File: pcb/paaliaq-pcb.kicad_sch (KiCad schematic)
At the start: 9 parts, among them J1 SODIMM-200, J2 HDMI_A, U1 W65C816SxP, U3 MCP1727-3302xSN

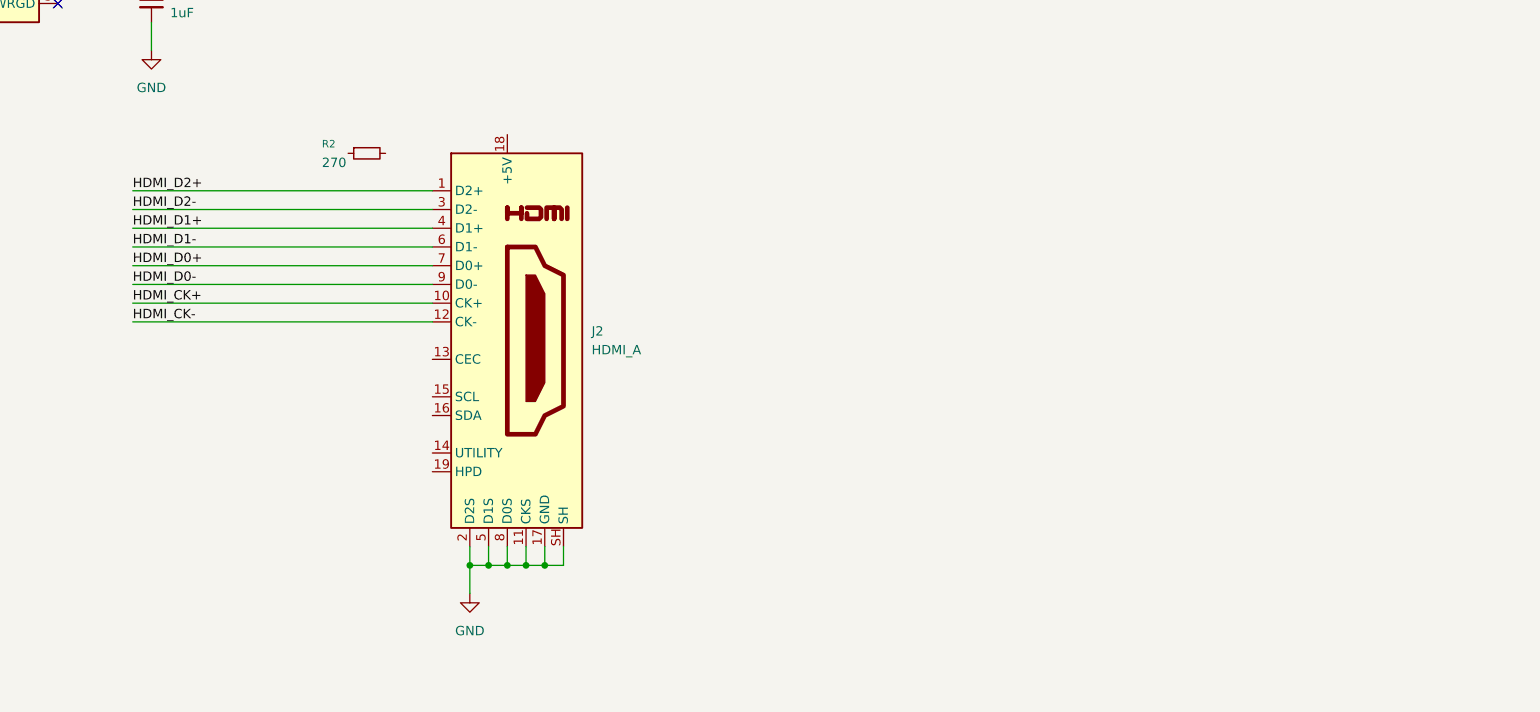
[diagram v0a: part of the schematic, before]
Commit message: wip dvi phy
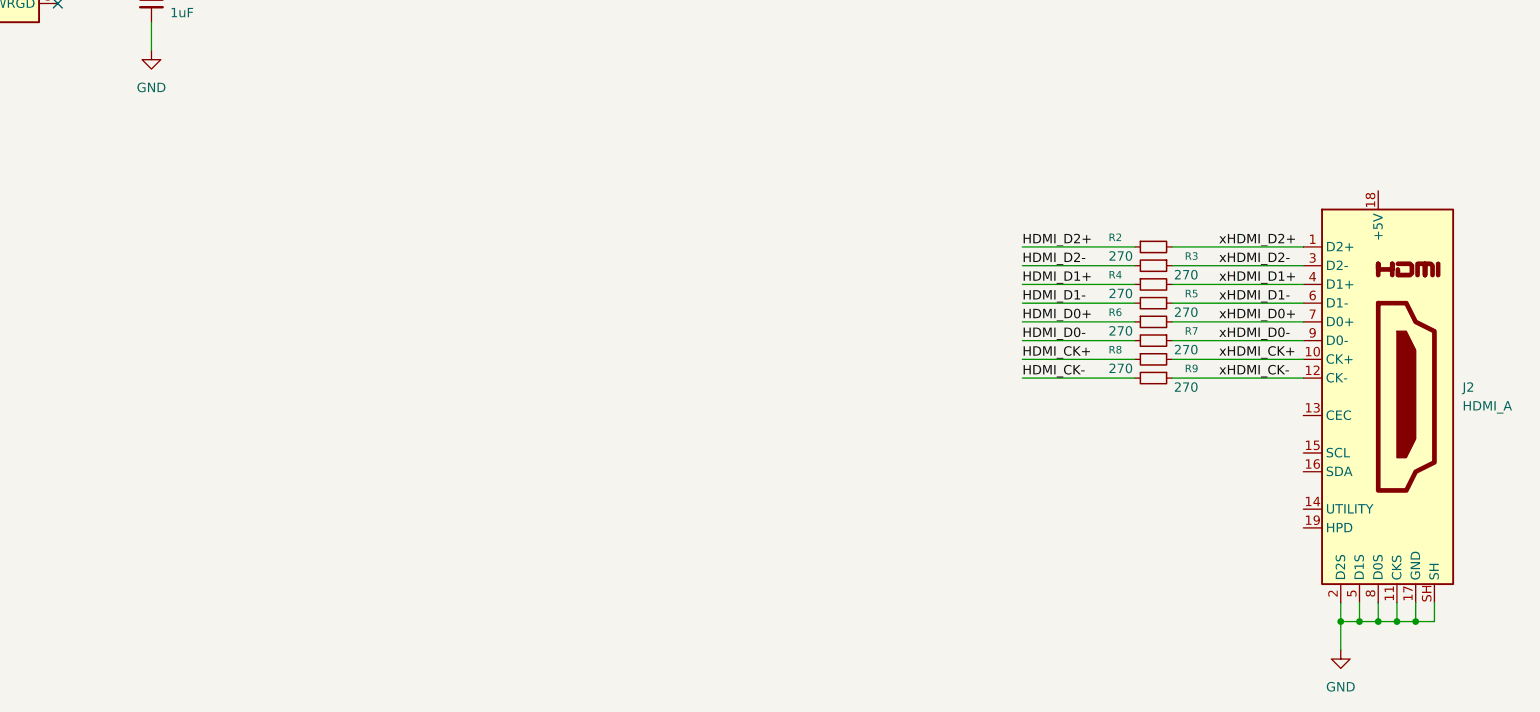
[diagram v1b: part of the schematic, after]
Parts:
- added R3, R4, R5, R6, R7, R8, R9: 270, Resistor_SMD:R_0603_1608Metric_Pad0.98x0.95mm_HandSolder, symbol Device:R_Small
- R2: footprint Resistor_SMD:R_0805_2012Metric_Pad1.20x1.40mm_HandSolder -> Resistor_SMD:R_0603_1608Metric_Pad0.98x0.95mm_HandSolder
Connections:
- net HDMI_CK+: now also R8.1; no longer J2.10 (CK+)
- net HDMI_CK-: now also R9.2; no longer J2.12 (CK-)
- net HDMI_D0+: now also R6.1; no longer J2.7 (D0+)
- net HDMI_D0-: now also R7.2; no longer J2.9 (D0-)
- net HDMI_D1+: now also R4.1; no longer J2.4 (D1+)
- net HDMI_D1-: now also R5.2; no longer J2.6 (D1-)
- net HDMI_D2+: now also R2.1; no longer J2.1 (D2+)
- net HDMI_D2-: now also R3.2; no longer J2.3 (D2-)
- net xHDMI_D2+: now reaches R2.2
- net xHDMI_D2+: now also J2.1 (D2+)
- new net xHDMI_CK+: J2.10 (CK+), R8.2
- new net xHDMI_CK-: J2.12 (CK-), R9.1
- new net xHDMI_D0+: J2.7 (D0+), R6.2
- new net xHDMI_D0-: J2.9 (D0-), R7.1
- new net xHDMI_D1+: J2.4 (D1+), R4.2
- new net xHDMI_D1-: J2.6 (D1-), R5.1
- new net xHDMI_D2-: J2.3 (D2-), R3.1
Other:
- moved on the sheet: J2, R2

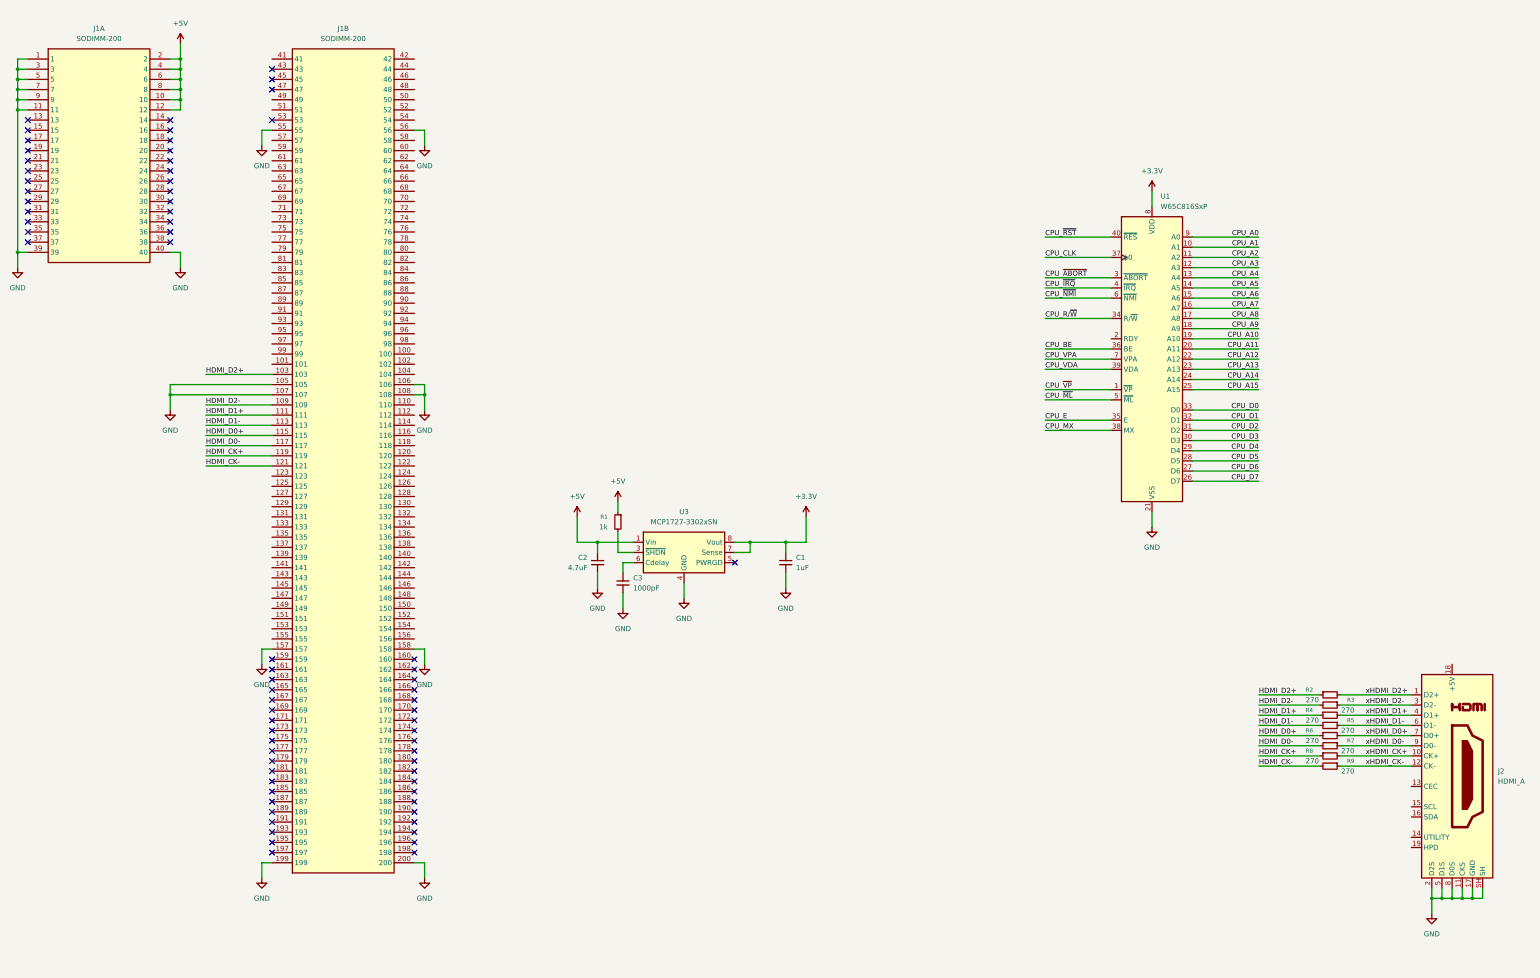
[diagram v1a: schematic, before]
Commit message: wip use resistor arrays and swap pairs and +/-
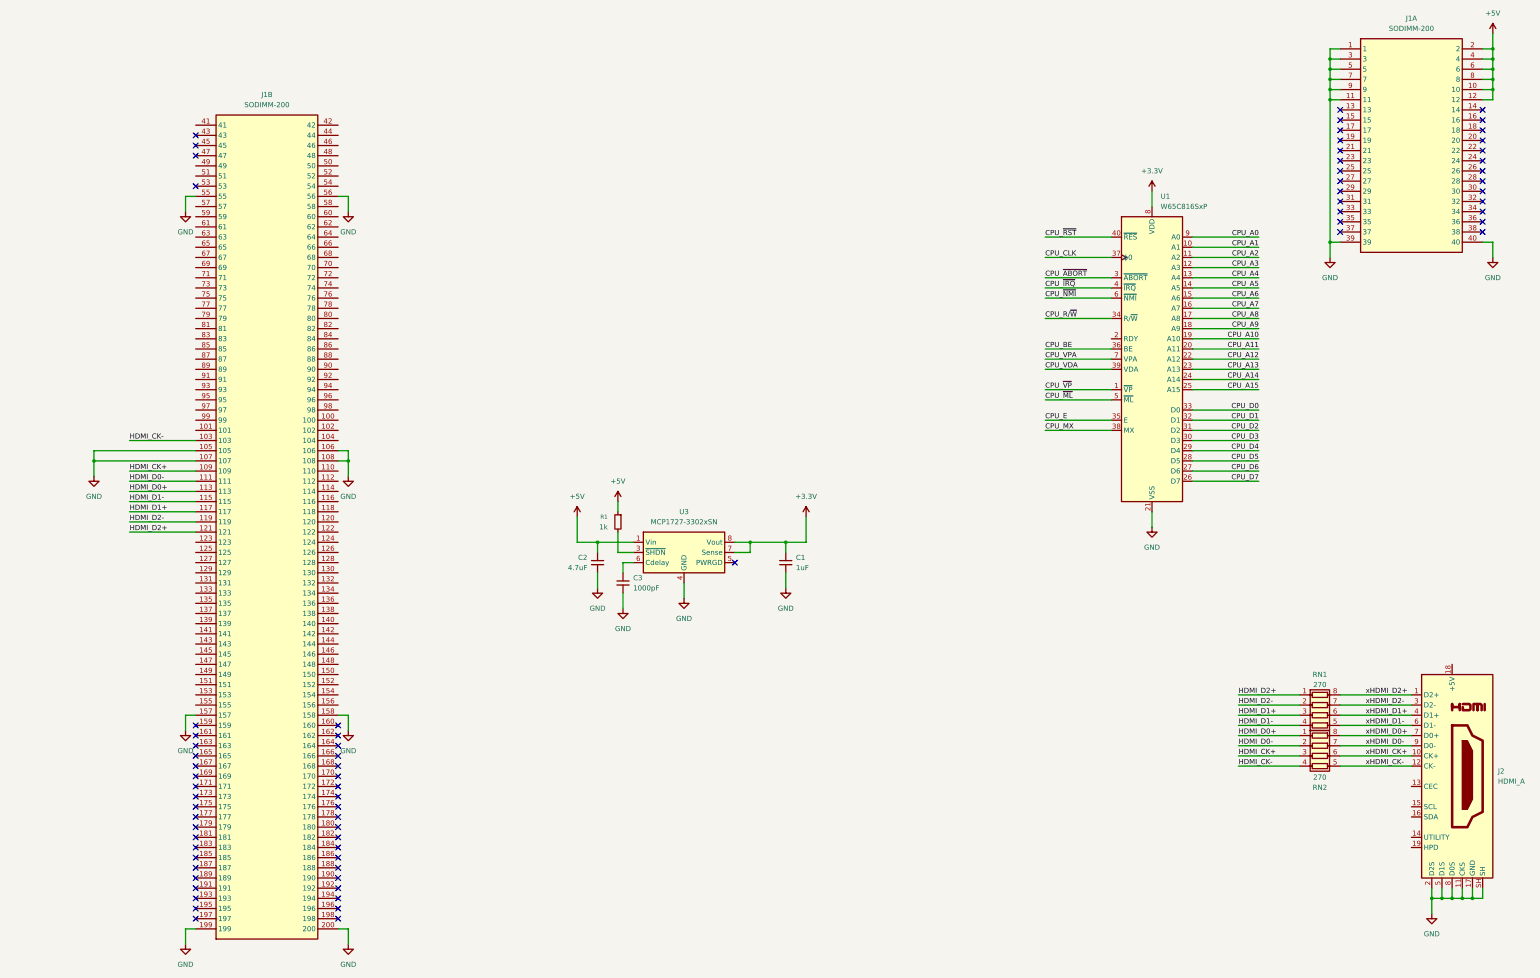
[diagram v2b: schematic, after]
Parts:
- removed R2, R3, R4, R5, R6, R7, R8, R9: 270, Resistor_SMD:R_0603_1608Metric_Pad0.98x0.95mm_HandSolder, symbol Device:R_Small
- added RN1, RN2: 270, Resistor_SMD:R_Array_Convex_4x1206, symbol Device:R_Pack04
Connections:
- net HDMI_CK+: now also J1.109, RN2.3 (R3.1); no longer J1.119
- net HDMI_CK-: now also J1.103, RN2.4 (R4.1); no longer J1.121
- net HDMI_D0+: now also J1.113, RN2.1 (R1.1); no longer J1.115
- net HDMI_D0-: now also J1.111, RN2.2 (R2.1); no longer J1.117
- net HDMI_D1+: now also J1.117, RN1.3 (R3.1); no longer J1.111
- net HDMI_D1-: now also J1.115, RN1.4 (R4.1); no longer J1.113
- net HDMI_D2+: now also J1.121, RN1.1 (R1.1); no longer J1.103
- net HDMI_D2-: now also J1.119, RN1.2 (R2.1); no longer J1.109
- net xHDMI_CK+: now also RN2.6 (R3.2)
- net xHDMI_CK-: now also RN2.5 (R4.2)
- net xHDMI_D0+: now also RN2.8 (R1.2)
- net xHDMI_D0-: now also RN2.7 (R2.2)
- net xHDMI_D1+: now also RN1.6 (R3.2)
- net xHDMI_D1-: now also RN1.5 (R4.2)
- net xHDMI_D2+: now also RN1.8 (R1.2)
- net xHDMI_D2-: now also RN1.7 (R2.2)
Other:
- moved on the sheet: J1A, J1B
